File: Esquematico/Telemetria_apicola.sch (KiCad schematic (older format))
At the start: 0 parts

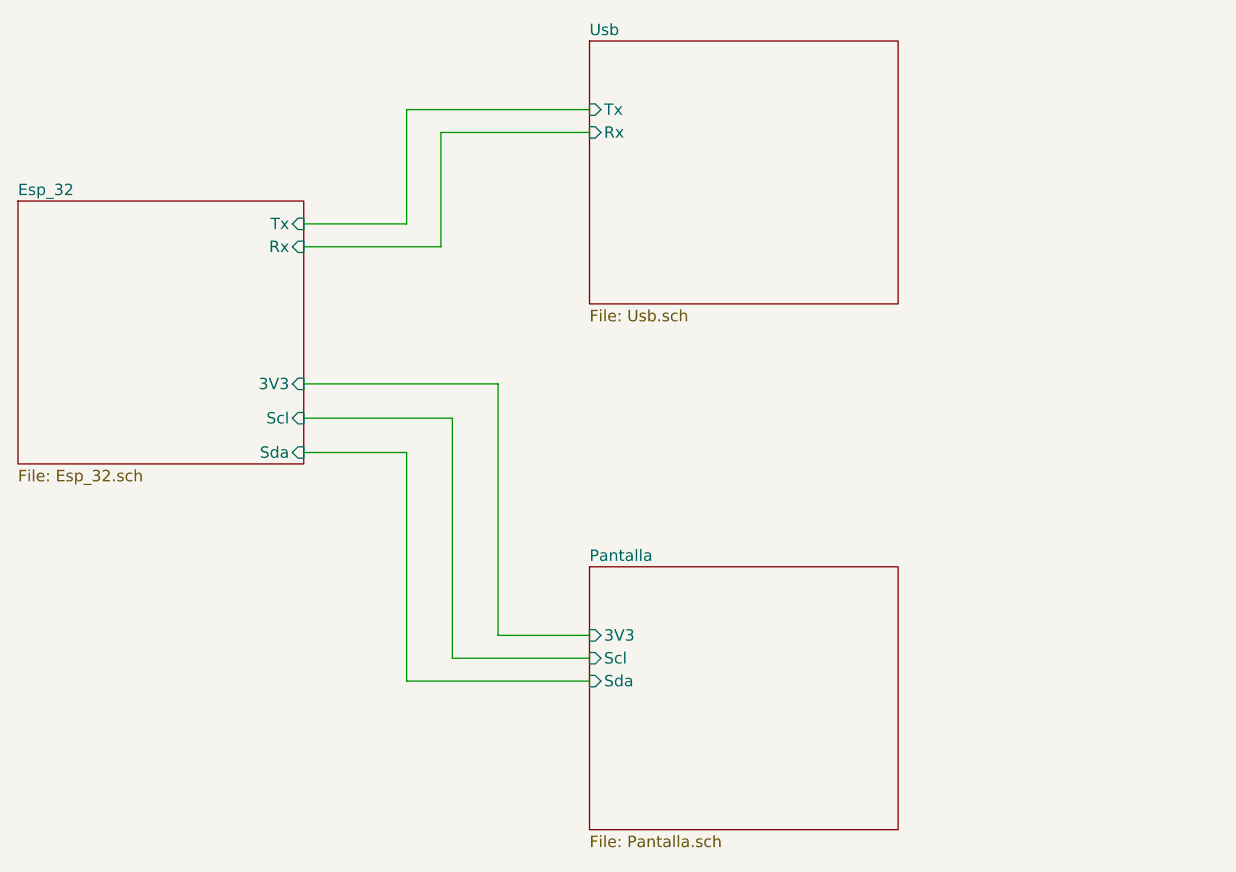
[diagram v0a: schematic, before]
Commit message: Add files via upload
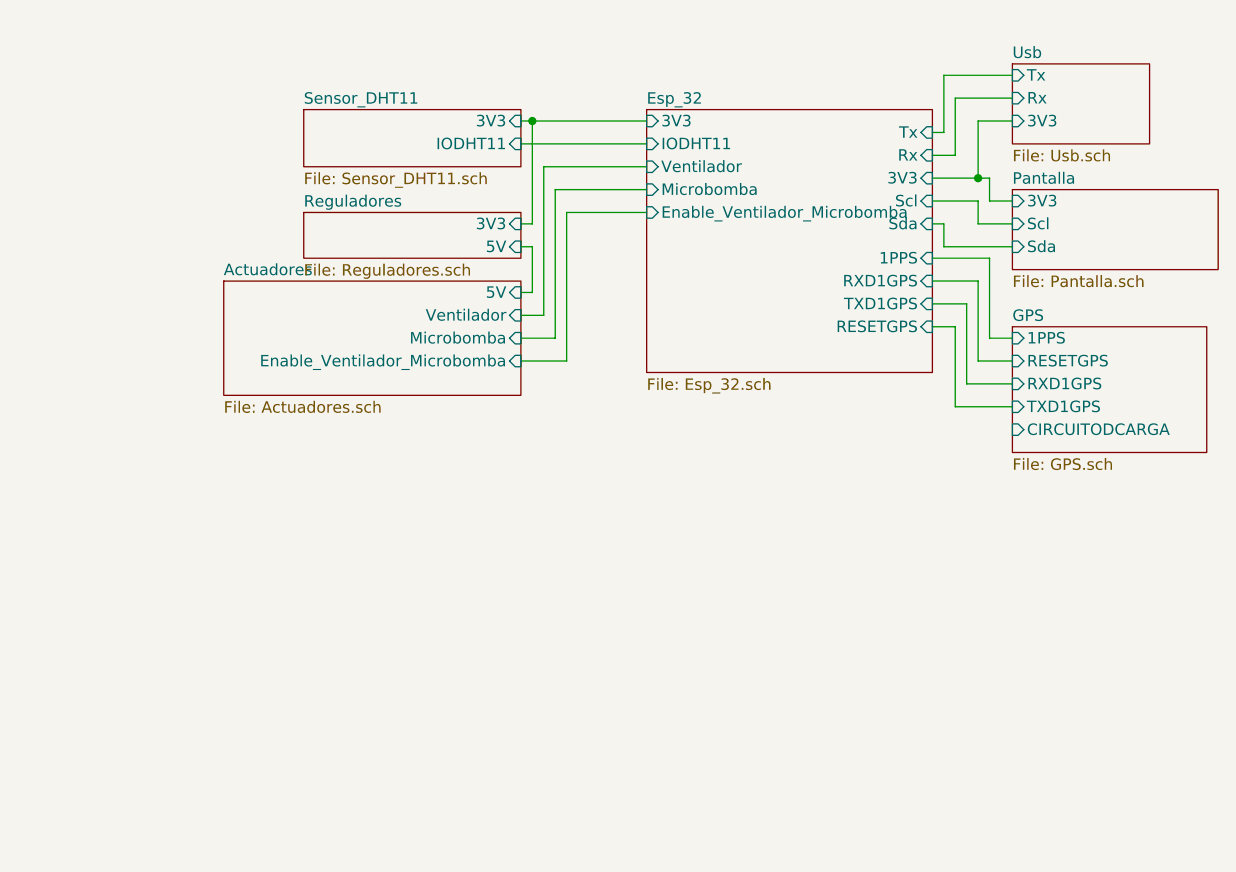
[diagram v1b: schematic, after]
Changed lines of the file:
@@
 $Descr A4 11693 8268
 encoding utf-8
-Sheet 1 4
+Sheet 1 8
 Title ""
 Date ""
@@
 $EndDescr
 $Sheet
-S 5150 2350 1350 1150
+S 7000 2450 600  350
 U 61A89954
 F0 "Usb" 50
 F1 "Usb.sch" 50
-F2 "Tx" I L 5150 2650 50
-F3 "Rx" I L 5150 2750 50
+F2 "Tx" I L 7000 2500 50
+F3 "Rx" I L 7000 2600 50
+F4 "3V3" I L 7000 2700 50
 $EndSheet
 $Sheet
-S 5150 4650 1350 1150
+S 7000 3000 900  350
 U 61A89771
 F0 "Pantalla" 50
 F1 "Pantalla.sch" 50
-F2 "3V3" I L 5150 4950 50
-F3 "Scl" I L 5150 5050 50
-F4 "Sda" I L 5150 5150 50
+F2 "3V3" I L 7000 3050 50
+F3 "Scl" I L 7000 3150 50
+F4 "Sda" I L 7000 3250 50
 $EndSheet
 $Sheet
-S 2650 3050 1250 1150
+S 5400 2650 1250 1150
 U 61A89555
 F0 "Esp_32" 50
 F1 "Esp_32.sch" 50
-F2 "Sda" I R 3900 4150 50
-F3 "Scl" I R 3900 4000 50
-F4 "3V3" I R 3900 3850 50
-F5 "Tx" I R 3900 3150 50
-F6 "Rx" I R 3900 3250 50
+F2 "Sda" I R 6650 3150 50
+F3 "Scl" I R 6650 3050 50
+F4 "3V3" I R 6650 2950 50
+F5 "Tx" I R 6650 2750 50
+F6 "Rx" I R 6650 2850 50
+F7 "IODHT11" I L 5400 2800 50
+F8 "3V3" I L 5400 2700 50
+F9 "Ventilador" I L 5400 2900 50
+F10 "Microbomba" I L 5400 3000 50
+F11 "Enable_Ventilador_Microbomba" I L 5400 3100 50
+F12 "1PPS" I R 6650 3300 50
+F13 "RXD1GPS" I R 6650 3400 50
+F14 "TXD1GPS" I R 6650 3500 50
+F15 "RESETGPS" I R 6650 3600 50
+$EndSheet
+$Sheet
+S 3900 2650 950  250
+U 61B54779
+F0 "Sensor_DHT11" 50
+F1 "Sensor_DHT11.sch" 50
+F2 "IODHT11" I R 4850 2800 50
+F3 "3V3" I R 4850 2700 50
 $EndSheet
 Wire Wire Line
-	3900 3850 4750 3850
+	4850 2700 4900 2700
 Wire Wire Line
-	4750 3850 4750 4950
+	4850 2800 5400 2800
+$Sheet
+S 3900 3100 950  200
+U 61B5A8A7
+F0 "Reguladores" 50
+F1 "Reguladores.sch" 50
+F2 "3V3" I R 4850 3150 50
+F3 "5V" I R 4850 3250 50
+$EndSheet
 Wire Wire Line
-	4750 4950 5150 4950
+	6650 2750 6700 2750
 Wire Wire Line
-	5150 5050 4550 5050
+	6700 2750 6700 2500
 Wire Wire Line
-	4550 5050 4550 4000
+	6700 2500 7000 2500
 Wire Wire Line
-	4550 4000 3900 4000
+	6650 2850 6750 2850
 Wire Wire Line
-	3900 4150 4350 4150
+	6750 2850 6750 2600
 Wire Wire Line
-	4350 4150 4350 5150
+	6750 2600 7000 2600
 Wire Wire Line
-	4350 5150 5150 5150
+	7000 2700 6850 2700
 Wire Wire Line
-	3900 3150 4350 3150
+	6850 2700 6850 2950
 Wire Wire Line
-	4350 3150 4350 2650
+	6850 2950 6650 2950
 Wire Wire Line
-	4350 2650 5150 2650
+	6650 3150 6700 3150
 Wire Wire Line
-	3900 3250 4500 3250
+	6700 3150 6700 3250
 Wire Wire Line
-	4500 3250 4500 2750
+	6700 3250 7000 3250
 Wire Wire Line
-	4500 2750 5150 2750
+	6850 3050 6850 3150
+Wire Wire Line
+	6850 3150 7000 3150
+Wire Wire Line
+	6650 3050 6850 3050
+Wire Wire Line
+	7000 3050 6900 3050
+Wire Wire Line
+	6900 3050 6900 2950
+Wire Wire Line
+	6900 2950 6850 2950
+Connection ~ 6850 2950
+Wire Wire Line
+	4900 3150 4850 3150
+Wire Wire Line
+	4900 3150 4900 2700
+Connection ~ 4900 2700
+Wire Wire Line
+	4900 2700 5400 2700
+$Sheet
+S 3550 3400 1300 500
+U 61B678E2
+F0 "Actuadores" 50
+F1 "Actuadores.sch" 50
+F2 "5V" I R 4850 3450 50
+F3 "Ventilador" I R 4850 3550 50
+F4 "Microbomba" I R 4850 3650 50
+F5 "Enable_Ventilador_Microbomba" I R 4850 3750 50
+$EndSheet
+Wire Wire Line
+	4850 3250 4900 3250
+Wire Wire Line
+	4950 2900 5400 2900
+Wire Wire Line
+	5400 3000 5000 3000
+Wire Wire Line
+	5050 3100 5400 3100
+Wire Wire Line
+	4850 3450 4900 3450
+Wire Wire Line
+	4900 3450 4900 3250
+Wire Wire Line
+	4950 2900 4950 3550
+Wire Wire Line
+	4950 3550 4850 3550
+Wire Wire Line
+	4850 3650 5000 3650
+Wire Wire Line
+	5000 3650 5000 3000
+Wire Wire Line
+	4850 3750 5050 3750
+Wire Wire Line
+	5050 3750 5050 3100
+$Sheet
+S 7000 3600 850  550
+U 61B777C0
+F0 "GPS" 50
+F1 "GPS.sch" 50
+F2 "1PPS" I L 7000 3650 50
+F3 "RESETGPS" I L 7000 3750 50
+F4 "RXD1GPS" I L 7000 3850 50
+F5 "TXD1GPS" I L 7000 3950 50
+F6 "CIRCUITODCARGA" I L 7000 4050 50
+$EndSheet
+Wire Wire Line
+	6650 3300 6900 3300
+Wire Wire Line
+	6900 3300 6900 3650
+Wire Wire Line
+	6900 3650 7000 3650
+Wire Wire Line
+	6650 3400 6850 3400
+Wire Wire Line
+	6850 3400 6850 3750
+Wire Wire Line
+	6850 3750 7000 3750
+Wire Wire Line
+	6650 3500 6800 3500
+Wire Wire Line
+	6800 3500 6800 3850
+Wire Wire Line
+	6800 3850 7000 3850
+Wire Wire Line
+	6650 3600 6750 3600
+Wire Wire Line
+	6750 3600 6750 3950
+Wire Wire Line
+	6750 3950 7000 3950
 $EndSCHEMATC
